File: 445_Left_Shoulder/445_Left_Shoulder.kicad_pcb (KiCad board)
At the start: 2 copper layers, 24.9 x 18 mm, 2 parts, among them J1 69167-107HLF, U1 LSM6DSMTR

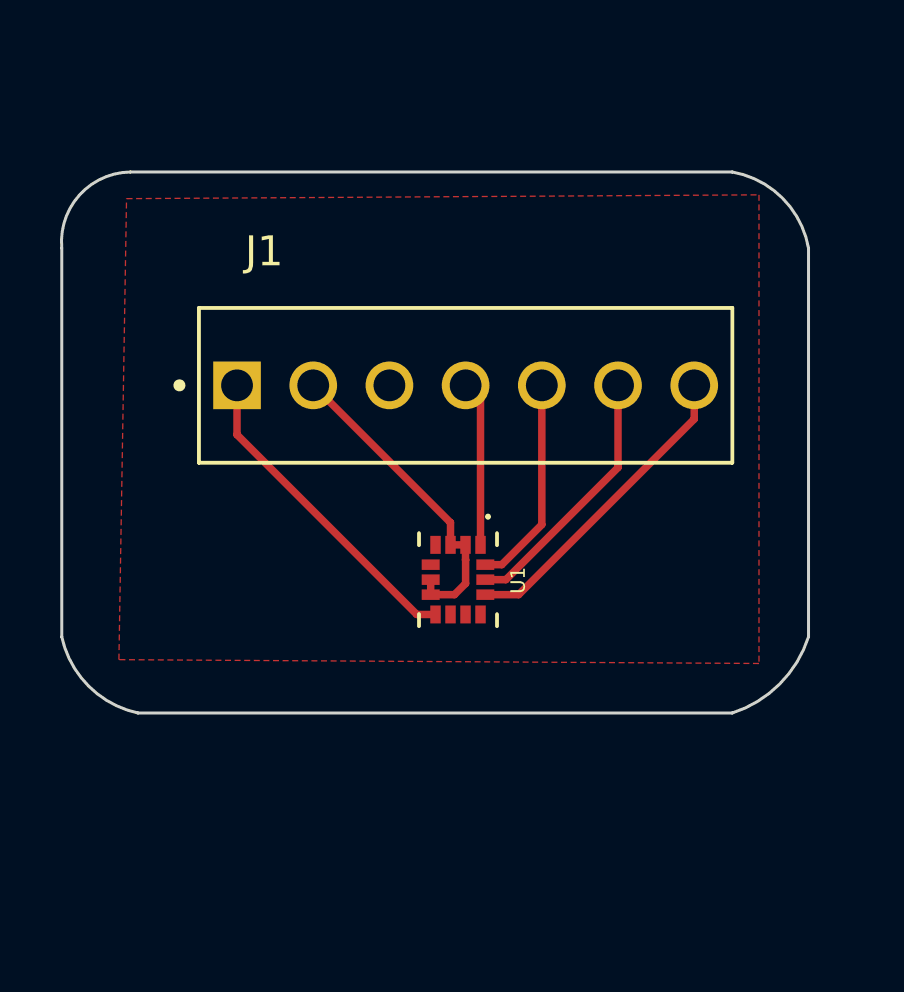
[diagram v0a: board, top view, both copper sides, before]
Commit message: Layout First Draft
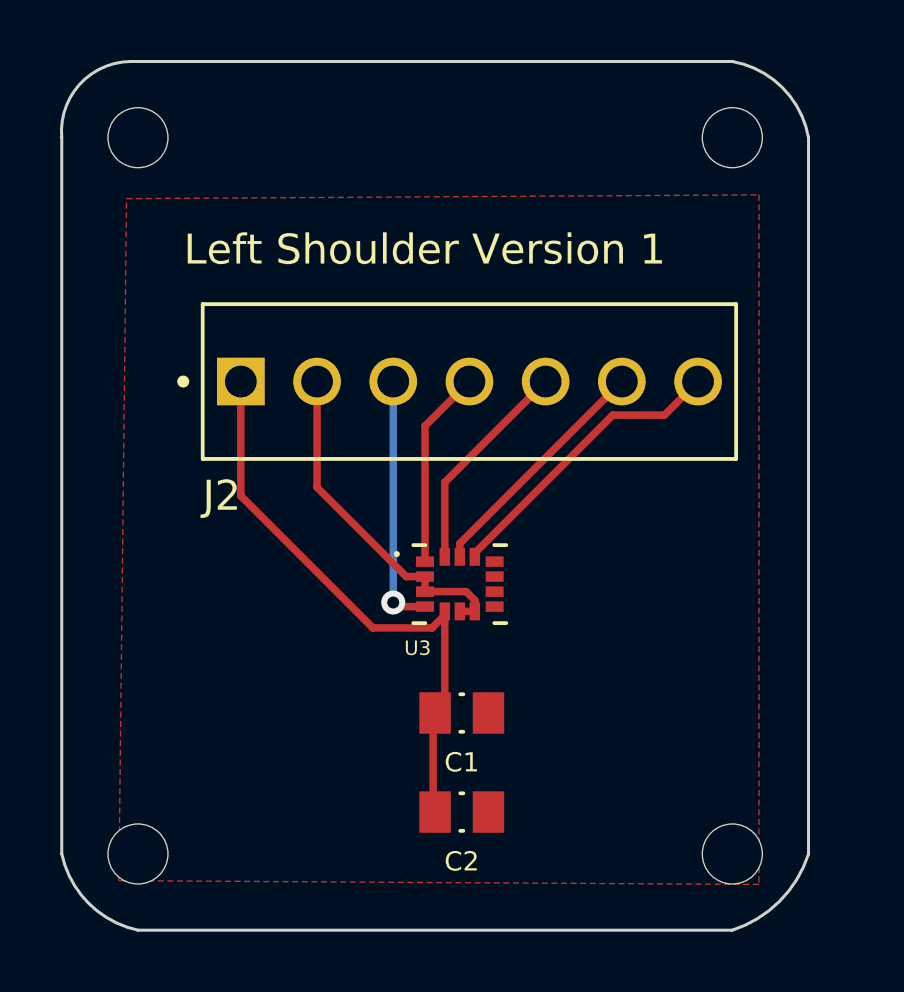
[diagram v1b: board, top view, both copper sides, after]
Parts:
- removed J1: 69167-107HLF, 69167-107HLF:AMPHENOL_69167-107HLF
- removed U1: LSM6DSMTR, LSM6DSMTR (1):PQFN50P300X250X86-14N
- added C1: 100nF, CL21F104ZAANNNC:CAPC2012X135N, F.Cu at (143.8, 97.0)
- added C2: 100nF, CL21F104ZAANNNC:CAPC2012X135N, F.Cu at (143.8, 100.3)
- added H1: MountingHole, MountingHole:MountingHole_2mm, F.Cu at (133.0, 77.9)
- added H2: MountingHole, MountingHole:MountingHole_2mm, F.Cu at (152.8, 77.9)
- added H3: MountingHole, MountingHole:MountingHole_2mm, F.Cu at (133.0, 101.7)
- added H4: MountingHole, MountingHole:MountingHole_2mm, F.Cu at (152.8, 101.7)
- added J2: 69167-107HLF, 69167-107HLF:AMPHENOL_69167-107HLF, F.Cu at (144.0, 86.0)
- added U3: LSM6DSMTR, LSM6DSMTR (1):PQFN50P300X250X86-14N, F.Cu at (143.7, 92.7)
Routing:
- net /CS0: track 10.5 -> 0.00 mm
- net /SENSOR_1: track 0.00 -> 9.93 mm
- net /CLK: track 8.71 -> 0.00 mm
- net +3.3V: track 10.7 -> 19.4 mm
- net /INT1_1: track 0.00 -> 8.48 mm, vias 0 -> 1
- net /CLK1: track 0.00 -> 8.08 mm
- net /MOSI_1: track 0.00 -> 7.23 mm
- net /MOSI: track 7.08 -> 0.00 mm
- net /MISO_1: track 0.00 -> 6.62 mm
- net /MISO: track 5.52 -> 0.00 mm
- net GND: track 10.8 -> 11.5 mm
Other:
- board size 24.9 x 18 mm -> 24.9 x 29 mm
- board text added: "Left Shoulder Version 1"
